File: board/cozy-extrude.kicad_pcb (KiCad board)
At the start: 2 copper layers, 7 parts, among them J1 RPi-Pico-Socket, J2 BME280, J3 PWM-Fan, J4 Heater-Switch, K1 HF46F_5-HS1, U1 ULN2003

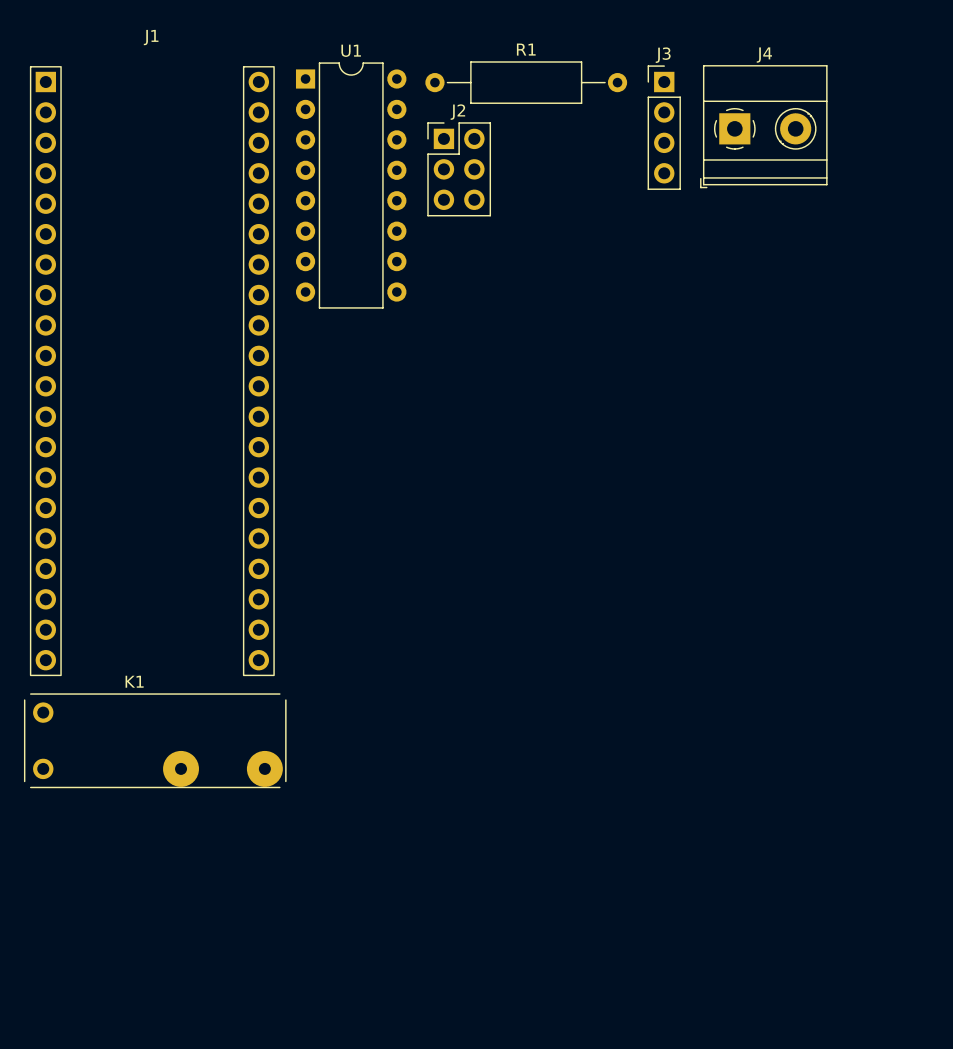
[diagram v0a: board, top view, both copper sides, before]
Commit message: pcb draft
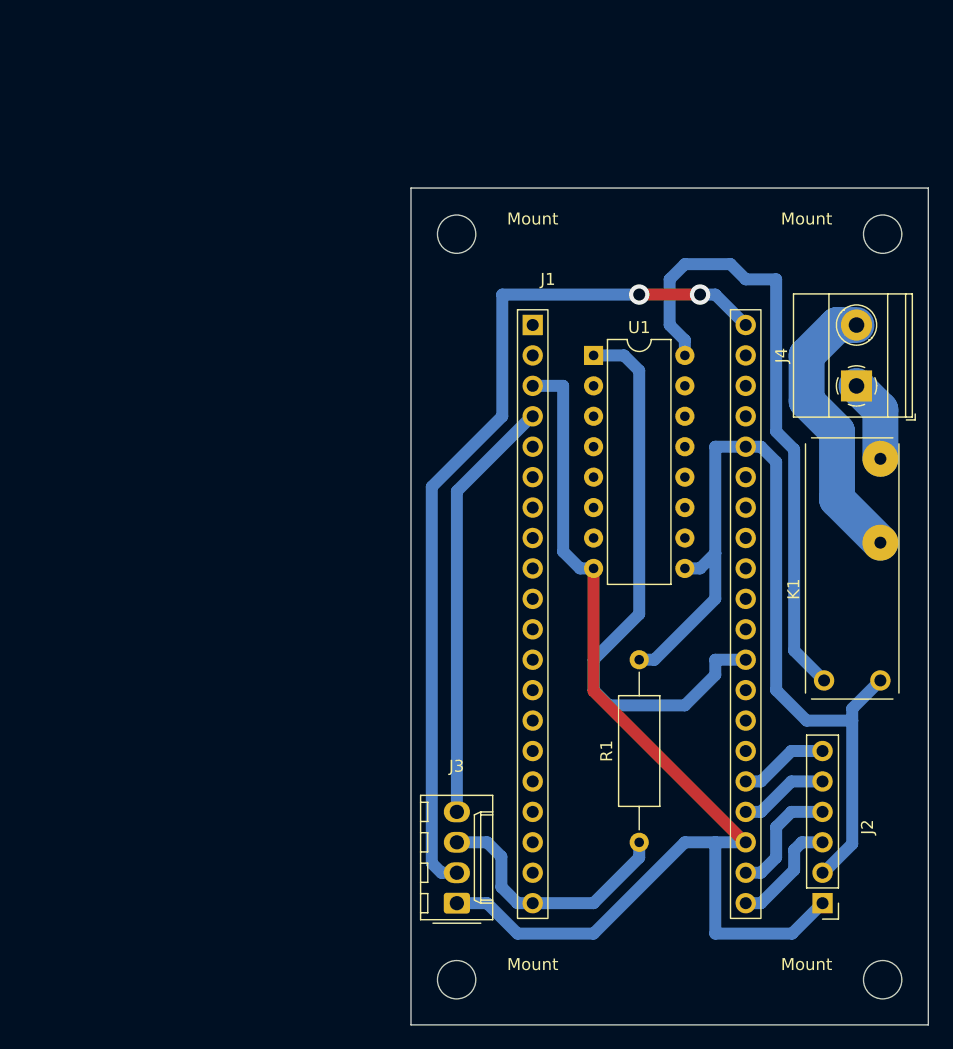
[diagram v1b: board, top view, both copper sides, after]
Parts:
- added Mount: MountingHole_3.2mm_M3, MountingHole:MountingHole_3.2mm_M3, F.Cu at (113.0, 128.3)
- added Mount: MountingHole_3.2mm_M3, MountingHole:MountingHole_3.2mm_M3, F.Cu at (148.6, 128.3)
- added Mount: MountingHole_3.2mm_M3, MountingHole:MountingHole_3.2mm_M3, F.Cu at (148.6, 66.0)
- added Mount: MountingHole_3.2mm_M3, MountingHole:MountingHole_3.2mm_M3, F.Cu at (113.0, 66.0)
- J2: footprint Connector_PinHeader_2.54mm:PinHeader_2x03_P2.54mm_Vertical -> Connector_PinHeader_2.54mm:PinHeader_1x06_P2.54mm_Vertical
- J3: footprint Connector_PinHeader_2.54mm:PinHeader_1x04_P2.54mm_Vertical -> Connector_Molex:Molex_KK-254_AE-6410-04A_1x04_P2.54mm_Vertical
- moved J2 71.2 mm to (143.6, 121.9), turned to 180 degrees
- moved J3 70.7 mm to (113.0, 121.9), turned to 90 degrees
- moved R1 65.7 mm to (128.3, 116.8), turned to 90 degrees
- moved K1 65.2 mm to (143.7, 103.3), turned to 90 degrees
- moved J1 45.4 mm to (119.4, 73.6)
- moved U1 33.3 mm to (124.5, 76.2)
- moved J4 23.7 mm to (146.4, 78.7), turned to 90 degrees
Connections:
- J1 pad 23: unconnected-(J1-Pad23) -> GND
- J1 pad 38: GND -> unconnected-(J1-Pad38)
- J4 pad 2: Net-(J4-Pad2) -> Net-(K1-Pad3)
- K1 pad 2: +3.3V -> +3V3
- K1 pad 3: Net-(J4-Pad1) -> Net-(K1-Pad3)
- K1 pad 4: Net-(J4-Pad2) -> Net-(J4-Pad1)
- U1 pad 9: +3.3V -> +3V3
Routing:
- net GND: track 0.00 -> 93.6 mm
- net +3V3: track 0.00 -> 74.4 mm
- net VBUS: track 0.00 -> 73.7 mm, vias 0 -> 2
- net Net-(K1-Pad1): track 0.00 -> 52.0 mm
- net /HEATER_EN: track 0.00 -> 48.1 mm
- net /PWM: track 0.00 -> 35.7 mm
- net Net-(K1-Pad3): track 0.00 -> 23.4 mm
- net /TACH: track 0.00 -> 21.7 mm
- net /CSB: track 0.00 -> 10.0 mm
- net /SDO: track 0.00 -> 9.49 mm
- net /SCL: track 0.00 -> 7.46 mm
- net /SDA: track 0.00 -> 7.46 mm
- net Net-(J4-Pad1): track 0.00 -> 6.98 mm
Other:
- board outline added: 43.2 x 69.9 mm
